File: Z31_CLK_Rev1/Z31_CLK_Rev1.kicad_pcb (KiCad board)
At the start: 2 copper layers, 74 x 50 mm, 16 parts, among them J1 Conn_01x06_Male, J2 ICSP, U1 MAX6922, U2 4BT-78Z_6L, U3 ATMEGA328-AURCT-ND, U4 MCP2510, U5 TJR1443, Y1 8MHz, Y2 16MHz

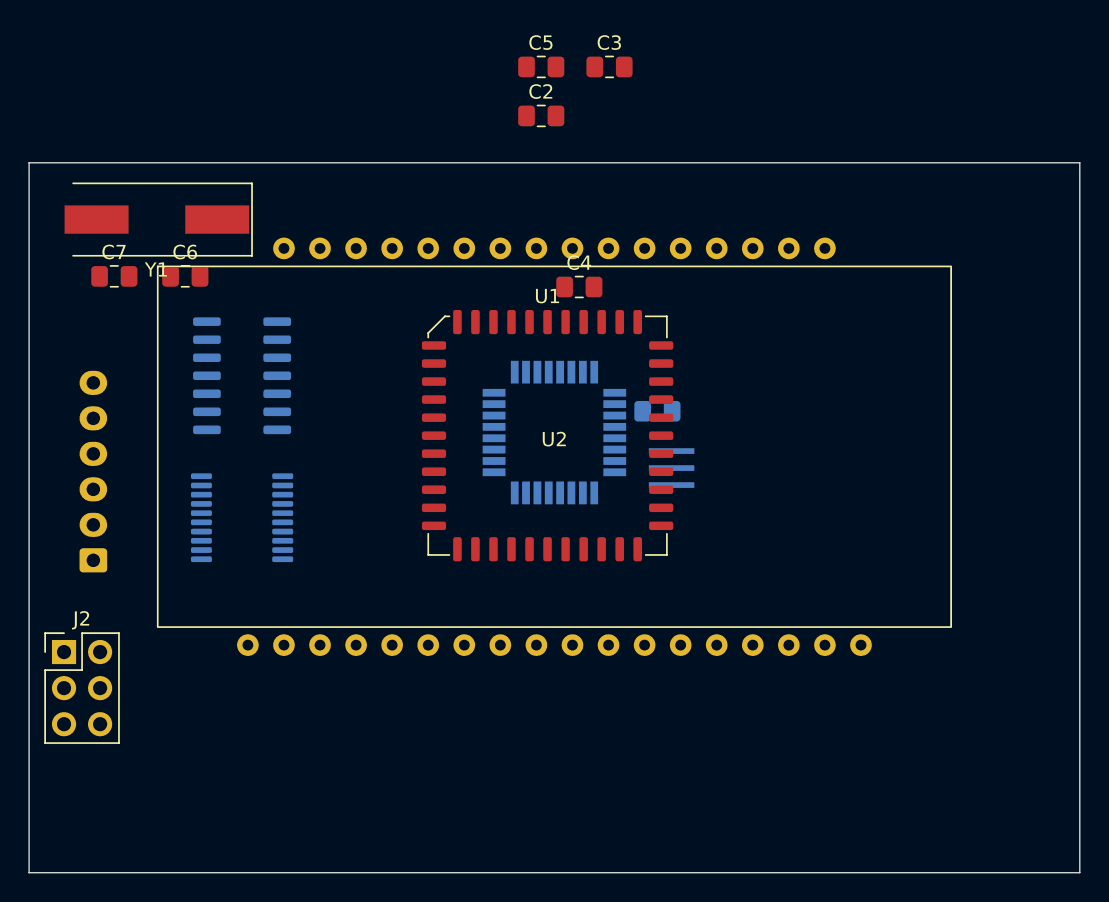
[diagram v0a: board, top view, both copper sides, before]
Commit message: add code
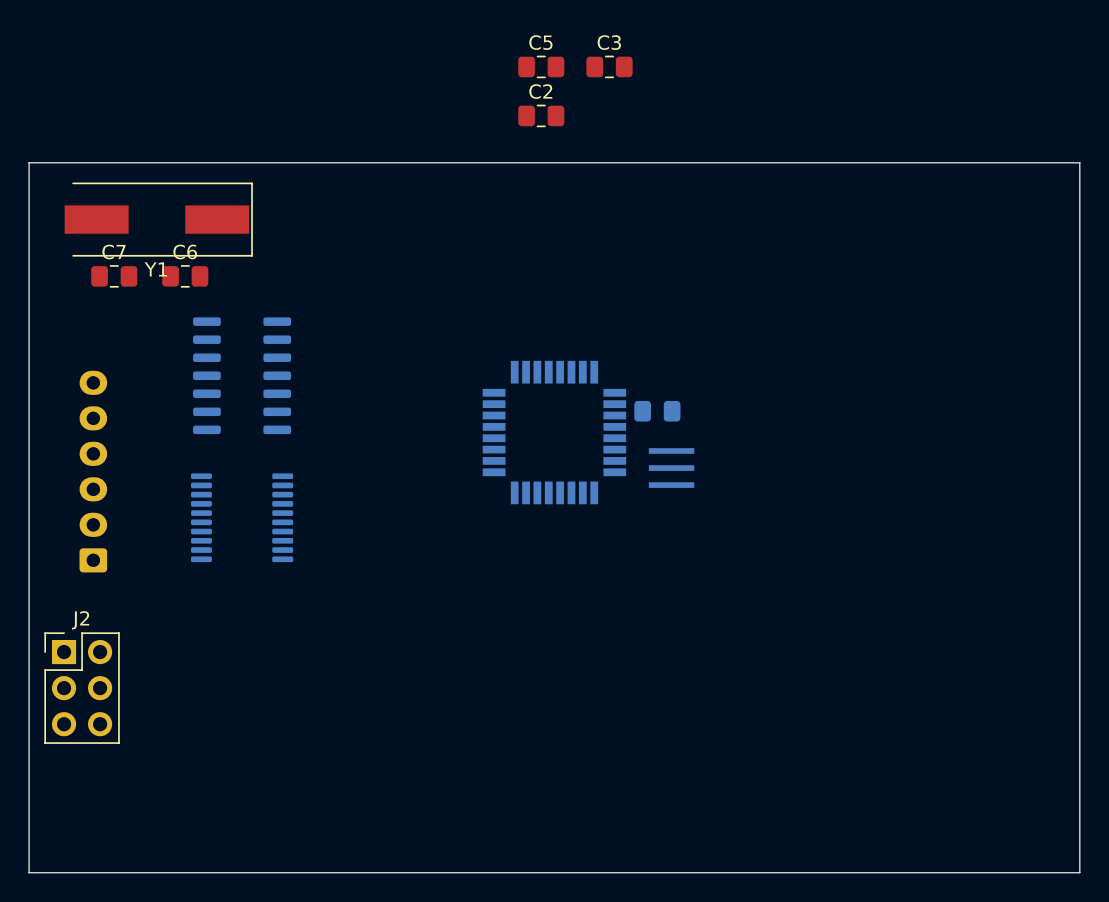
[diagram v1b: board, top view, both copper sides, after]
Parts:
- removed C4: 100n, Capacitor_SMD:C_0805_2012Metric_Pad1.18x1.45mm_HandSolder
- removed U1: MAX6922, Package_LCC:PLCC-44_16.6x16.6mm_P1.27mm
- removed U2: 4BT-78Z_6L, Personal:4BT-78Z_6L
